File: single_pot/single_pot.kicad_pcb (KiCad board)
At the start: 2 copper layers, 22 x 18 mm, 6 parts, among them J1 I/O connector

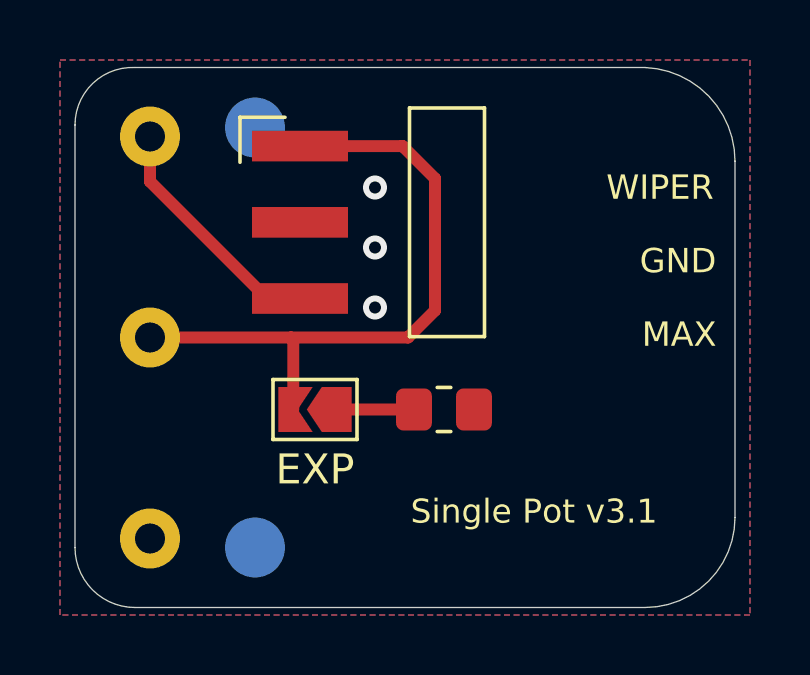
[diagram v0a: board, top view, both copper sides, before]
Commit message: Update to v3.1
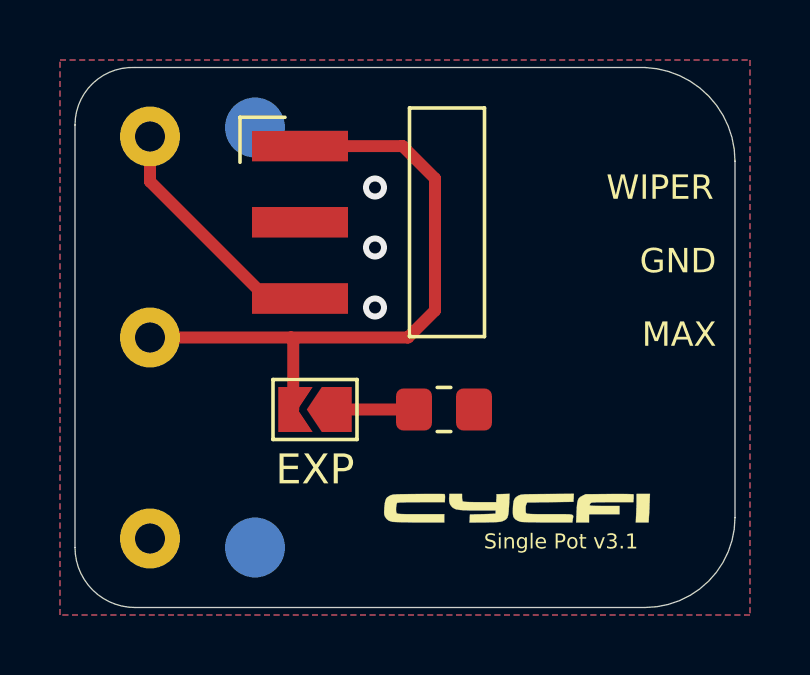
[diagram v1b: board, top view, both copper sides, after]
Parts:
- added G***: LOGO, cycfi_library:cycfi-logo-9mm, F.Cu at (150.7, 85.7)
- R1: value 4.7k -> 100k
